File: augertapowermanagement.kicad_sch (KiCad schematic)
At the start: 27 parts, among them J1 Screw_Terminal_01x02, J10 Screw_Terminal_01x10, J11 Screw_Terminal_01x10, J12 gnd block, J2 76825-0002, J3 USB_A_Stacked, J4 USB_A_Stacked, J5 USB_A_Stacked, J6 USB_A_Stacked, J7 Screw_Terminal_01x08, J8 Screw_Terminal_01x10, J9 5v block, K1 J107F1CS203VDC.80, Q1 IRF6623, SW1 SW_SPDT, U1 LM2596_5v, U2 ESP32-DEVKITC-32D, U24 MCP9808_MSOP

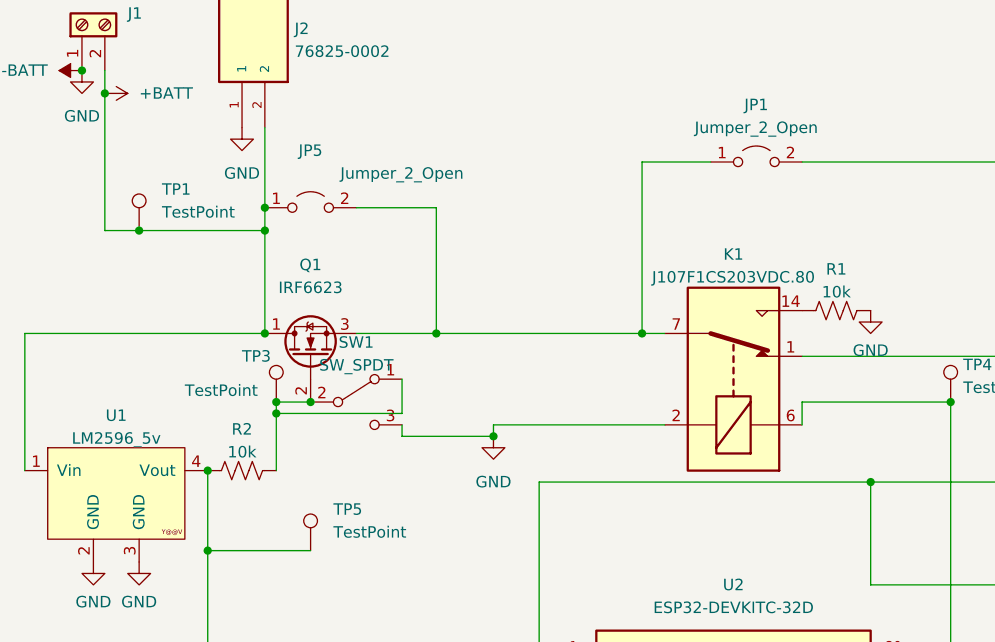
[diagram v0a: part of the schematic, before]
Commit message: update
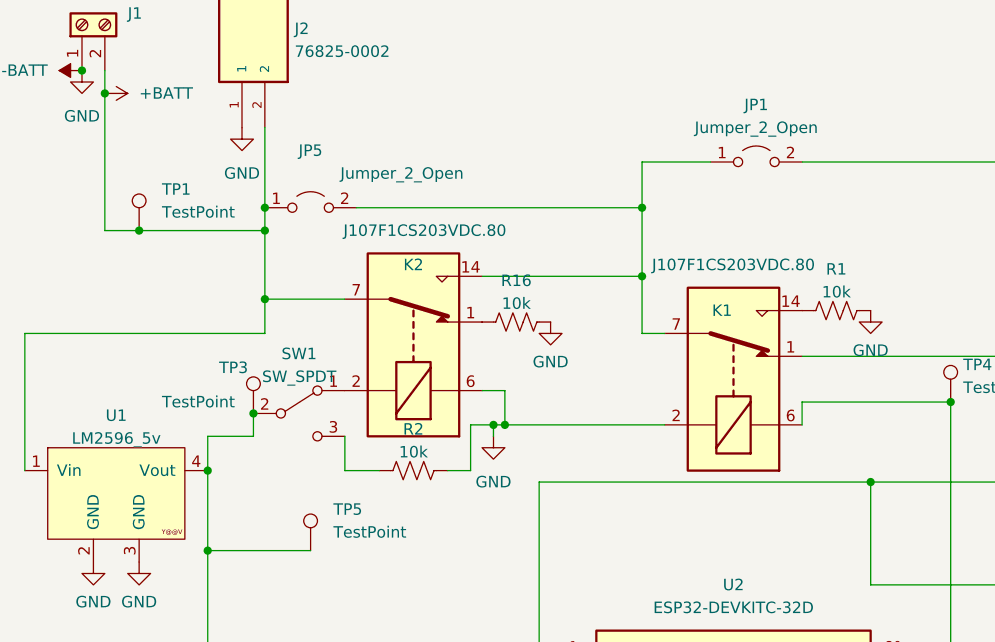
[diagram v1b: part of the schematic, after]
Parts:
- removed Q1: IRF6623, Package_DirectFET:DirectFET_ST, symbol Transistor_FET:IRF6623
- added K2: J107F1CS203VDC.80, cit:Relay_J107F, symbol Relay:DIPxx-1Cxx-51x
- added R16: 10k, Resistor_SMD:R_1210_3225Metric_Pad1.30x2.65mm_HandSolder, symbol Device:R_US
- TP1, TP3, TP4, TP5: Purchase (none) -> JUST PAD
- U24: Purchase (none) -> IN LAB
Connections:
- net +BATT: now also K2.7
- net -BATT: now also R2.1, K2.6, R16.2; no longer SW1.3 (C)
- net at C2.1, J9.1 (Pin_1), J9.2 (Pin_2)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: now also SW1.2 (B), TP3.1; no longer R2.1
- net at JP1.1 (A), JP5.2 (B), K1.7: now also K2.14; no longer K1.8
- new net: K2.1, R16.1
- new net: K2.2, SW1.1 (A)
- new net: R2.2, SW1.3 (C)
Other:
- moved on the sheet: R2, SW1, TP3
